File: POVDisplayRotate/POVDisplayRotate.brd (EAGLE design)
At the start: 80 x 99 mm, 34 parts, among them IC1 317EMP

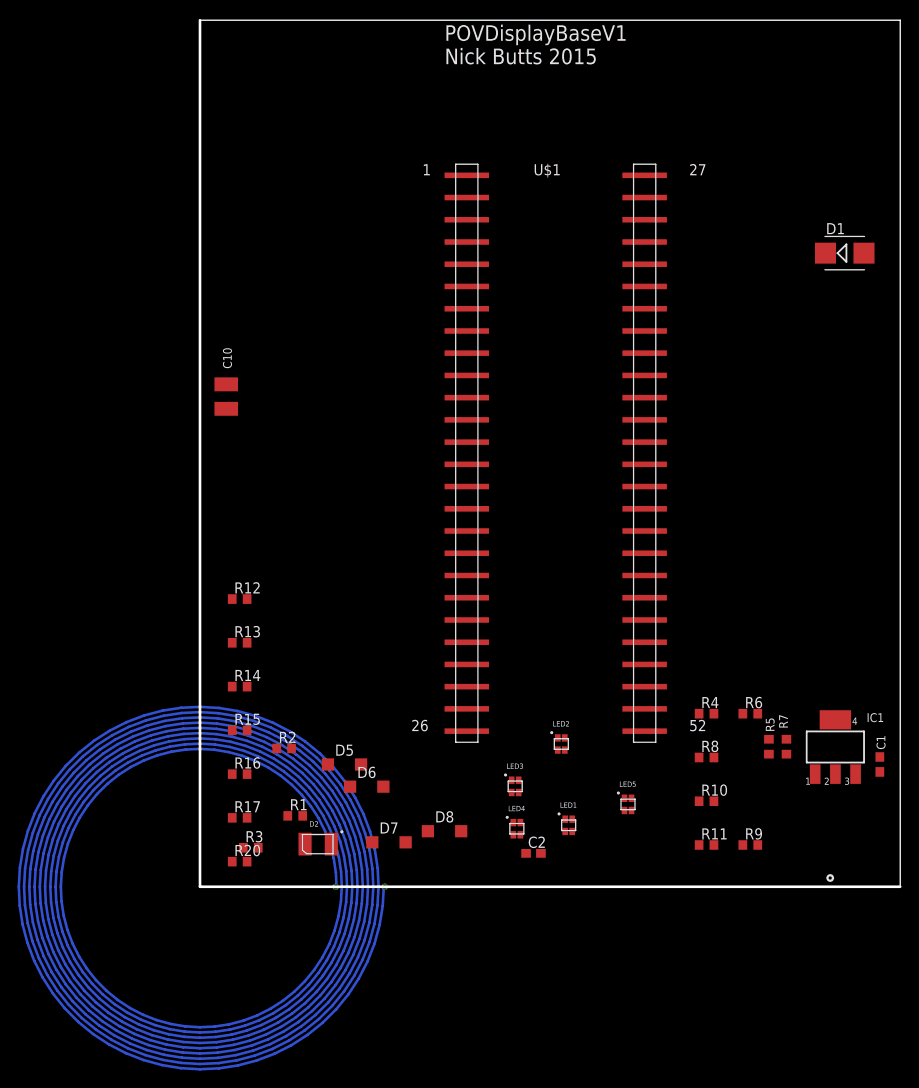
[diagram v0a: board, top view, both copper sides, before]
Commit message: Not sure what I updated.
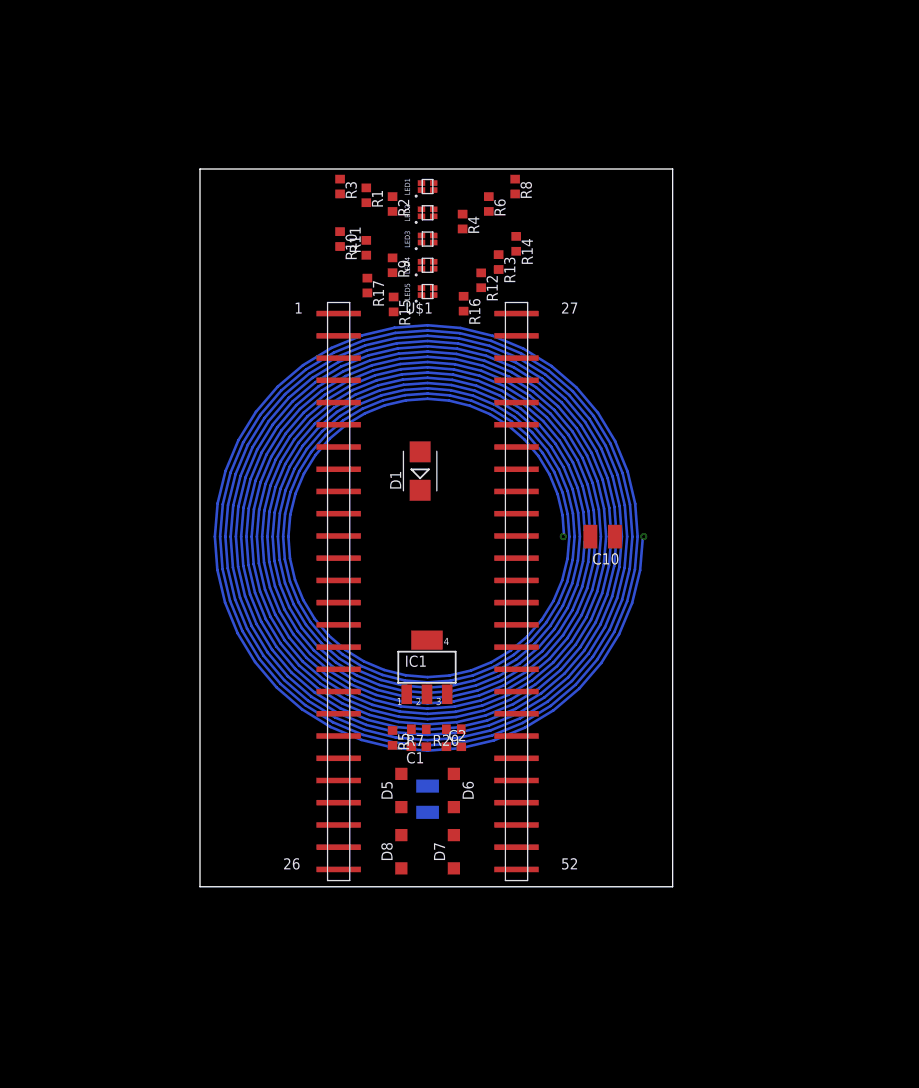
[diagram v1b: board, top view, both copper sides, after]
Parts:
- moved R11 78.5 mm to (19.0, 73.0), turned to 90 degrees
- moved R9 77.8 mm to (22.0, 71.0), turned to 270 degrees
- moved R10 76.7 mm to (16.0, 74.0), turned to 270 degrees
- moved R3 76.2 mm to (16.0, 80.0), turned to 270 degrees
- moved LED1 74.7 mm to (26.0, 80.0), turned to 90 degrees
- moved R1 71.4 mm to (19.0, 79.0), turned to 270 degrees
- moved R8 68.8 mm to (36.0, 80.0), turned to 270 degrees
- moved R6 65.4 mm to (33.0, 78.0), turned to 270 degrees
- moved LED4 65.2 mm to (26.0, 71.0), turned to 90 degrees
- moved R2 63.4 mm to (22.0, 78.0), turned to 270 degrees
- moved LED3 63.3 mm to (26.0, 74.0), turned to 90 degrees
- moved LED5 62.9 mm to (26.0, 68.0), turned to 90 degrees
- moved R4 62.8 mm to (30.0, 76.0), turned to 270 degrees
- moved LED2 62.6 mm to (26.0, 77.0), turned to 90 degrees
- moved R17 62.5 mm to (19.1, 68.7), turned to 270 degrees
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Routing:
- net N$19: track 0.00 -> 1892.7 mm, vias 0 -> 2
- net N$1: track 1034.6 -> 0.00 mm, vias 2 -> 0
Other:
- board size 80 x 99 mm -> 54 x 82 mm
- board text removed: "POVDisplayBaseV1 Nick Butts 2015"
